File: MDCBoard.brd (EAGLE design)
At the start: 43.9 x 32.6 mm, 200 parts, among them J1 JUMPER-SOLDER, J10 MICROSD-SOCKET, J11 USB-C-RECEPTACLE-KOREANHRO, J2 JUMPER-SOLDER, J3 JUMPER-SOLDER, J4 JUMPER-SOLDER, J5 JST-SM02B-SRSS-TB, J6 JUMPER-SOLDER, J7 JUMPER-SOLDER, J8 JUMPER-SOLDER, Q1 PMOS-NEXPERIA-SOT1220, Q2 PMOS-NEXPERIA-SOT1220, Q3 PMOS-NEXPERIA-SOT1220, Q4 DIODESINC-DMG2305UX, Q5 DIODESINC-DMG2305UX, Q6 DIODESINC-DMG2305UX, Q7 DIODESINC-DMG2305UX, Q8 DIODESINC-DMG2305UX, U1 TI-TPS2116, U10 TI-TPS22919DCK, U11 TI-TPS22919DCK, U12 TI-TPS22919DCK, U13 TI-TPS22919DCK, U14 TI-MSP430FR2422IRHL, U16 TI-TXB0102, U17 PANASONIC-EKMB110711X, U18 LATTICE-ICE40HX4K-BG121, U19 WINBOND-W25Q40EW, U2 DIODESINC-AP7350, U20 NEXPERIA-74LVC1G98-OR-INV-INP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, U21 NEXPERIA-74LVC1G98-BUFFER, U22 ON-AR0330CS1C12SPKA0, U23 ALLIANCE-AS4C8M16MSA-6BIN, U24 STM-STM32F730, U25 DIODESINC-DT1446-04V-7, U26 NEXPERIA-74LVC1G98-INVERTER, U3 NEXPERIA-74LVC1G98-NOR, U4 MICROCHIP-MCP7383X, U5 NEXPERIA-74LVC1G98-INVERTER, U6 EATON-STN101, U7 TI-TPS62A01, U8 TI-TPS62A01, U9 TI-TPS62A01, X1 EPSON-FC-135, X2 SITIME-SIT8021, X3 SITIME-SIT8021

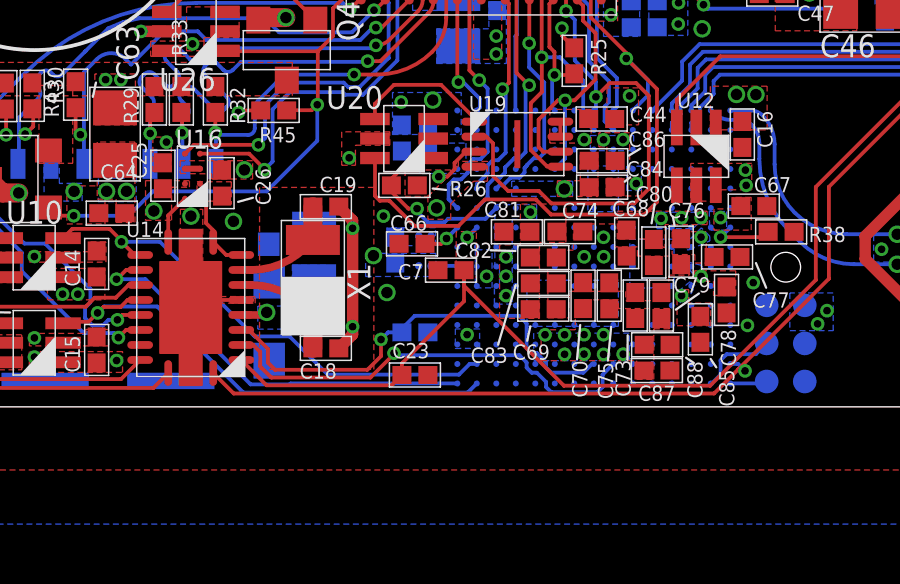
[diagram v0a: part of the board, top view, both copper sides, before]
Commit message: 13 airwires
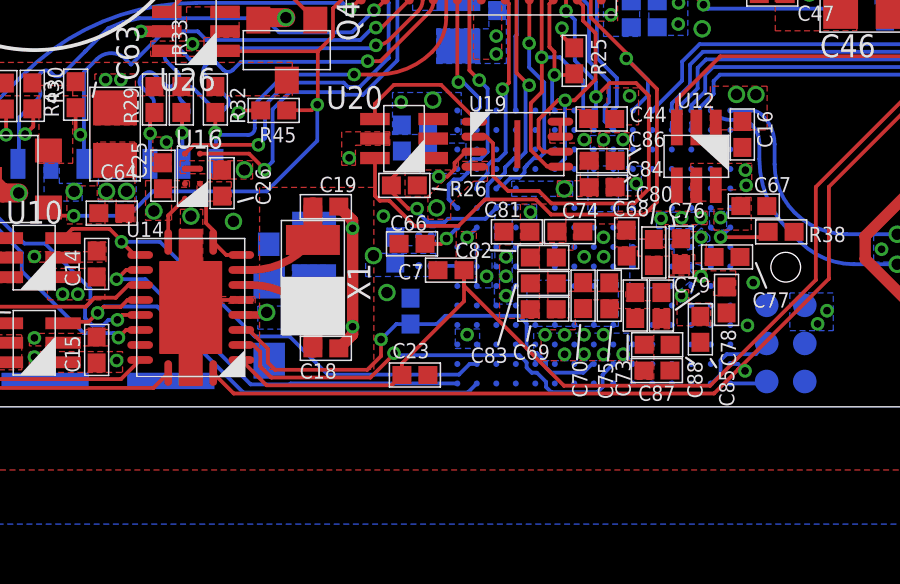
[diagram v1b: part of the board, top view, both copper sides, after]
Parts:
- moved C22 0.72 mm to (18.8, 3.19), turned to 90 degrees
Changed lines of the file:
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@@
 <attribute name="PN" value="MSP430FR2422IRHL" x="11.493478125" y="3.312359375" size="1.778" layer="27" rot="R180" display="off"/>
 </element>
-<element name="C22" library="EagleLibrary" package="0402" value="22p" x="18.96683125" y="2.48265625" smashed="yes" rot="MR180">
-<attribute name="MFG" value="Murata" x="18.96683125" y="2.48265625" size="1.778" layer="28" rot="MR180" display="off"/>
-<attribute name="NAME" x="20.983971875" y="2.391475" size="0.508" layer="26" font="vector" rot="MR0"/>
-<attribute name="PN" value="GRM1555C1H220JA01D" x="18.96683125" y="2.48265625" size="1.778" layer="28" rot="MR180" display="off"/>
+<element name="C22" library="EagleLibrary" package="0402" value="22p" x="18.8195125" y="3.191315625" smashed="yes" rot="MR90">
+<attribute name="MFG" value="Murata" x="18.8195125" y="3.191315625" size="1.778" layer="28" rot="MR90" display="off"/>
+<attribute name="NAME" x="18.91069375" y="5.20845625" size="0.508" layer="26" font="vector" rot="MR270"/>
+<attribute name="PN" value="GRM1555C1H220JA01D" x="18.8195125" y="3.191315625" size="1.778" layer="28" rot="MR90" display="off"/>
 </element>
 <element name="U10" library="EagleLibrary" package="TI-TPS22919DCK" value="TI-TPS22919DCK" x="6.27481875" y="4.97388125" smashed="yes" rot="R180">
@@
 <wire x1="29.2735" y1="28.2537375" x2="28.916" y2="29.437740625" width="0" layer="19" extent="1-16"/>
 <wire x1="21.93470625" y1="5.83590625" x2="21.030403125" y2="4.67901875" width="0" layer="19" extent="1-16"/>
-<wire x1="19.39933125" y1="2.48265625" x2="18.034" y2="3.81" width="0" layer="19" extent="16-16"/>
-<wire x1="19.398978125" y1="1.0617125" x2="19.39933125" y2="2.48265625" width="0" layer="19" extent="1-16"/>
 <wire x1="30.695915625" y1="6.69100625" x2="29.8034625" y2="4.99618125" width="0" layer="19" extent="1-1"/>
 <wire x1="28.346978125" y1="9.3113625" x2="29.8810375" y2="8.646903125" width="0" layer="19" extent="1-1"/>
+<wire x1="19.398978125" y1="1.0617125" x2="18.8195125" y2="3.623815625" width="0" layer="19" extent="1-16"/>
 </signal>
 <signal name="ICE_IMG_CLK16MHZ">
@@
 <wire x1="14.3030375" y1="1.2351625" x2="17.381546875" y2="1.2351625" width="0.127" layer="1"/>
 <contactref element="U24" pad="B8"/>
-<wire x1="18.53433125" y1="2.48265625" x2="18.074196875" y2="2.48265625" width="0.127" layer="16"/>
-<wire x1="18.074196875" y1="2.48265625" x2="17.836896875" y2="2.24535625" width="0.127" layer="16"/>
-<wire x1="18.961503125" y1="3.0342875" x2="18.53433125" y2="2.607115625" width="0.127" layer="16"/>
-<wire x1="18.53433125" y1="2.48265625" x2="18.53433125" y2="2.607115625" width="0.127" layer="16"/>
 <wire x1="22.68990625" y1="1.9586875" x2="22.860075" y2="1.78851875" width="0.127" layer="16"/>
 <wire x1="23.33990625" y1="1.3086875" x2="23.510075" y2="1.13851875" width="0.127" layer="16"/>
@@
 <wire x1="22.4359625" y1="3.0342875" x2="22.68990625" y2="2.78034375" width="0.127" layer="16"/>
 <wire x1="22.68990625" y1="2.78034375" x2="22.68990625" y2="1.9586875" width="0.127" layer="16"/>
-<wire x1="18.961503125" y1="3.0342875" x2="22.4359625" y2="3.0342875" width="0.127" layer="16"/>
+<wire x1="19.977503125" y1="3.0342875" x2="22.4359625" y2="3.0342875" width="0.127" layer="16"/>
+<wire x1="19.977503125" y1="3.0342875" x2="19.70203125" y2="2.758815625" width="0.127" layer="16"/>
+<wire x1="19.70203125" y1="2.758815625" x2="18.8195125" y2="2.758815625" width="0.127" layer="16"/>
+<wire x1="18.35035625" y1="2.758815625" x2="18.8195125" y2="2.758815625" width="0.127" layer="16"/>
+<wire x1="17.836896875" y1="2.24535625" x2="18.35035625" y2="2.758815625" width="0.127" layer="16"/>
 </signal>
 <signal name="ICE_MSP_SPI_DATA_X">
